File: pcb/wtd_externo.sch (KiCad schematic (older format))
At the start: 2 parts, among them U4 STWD100

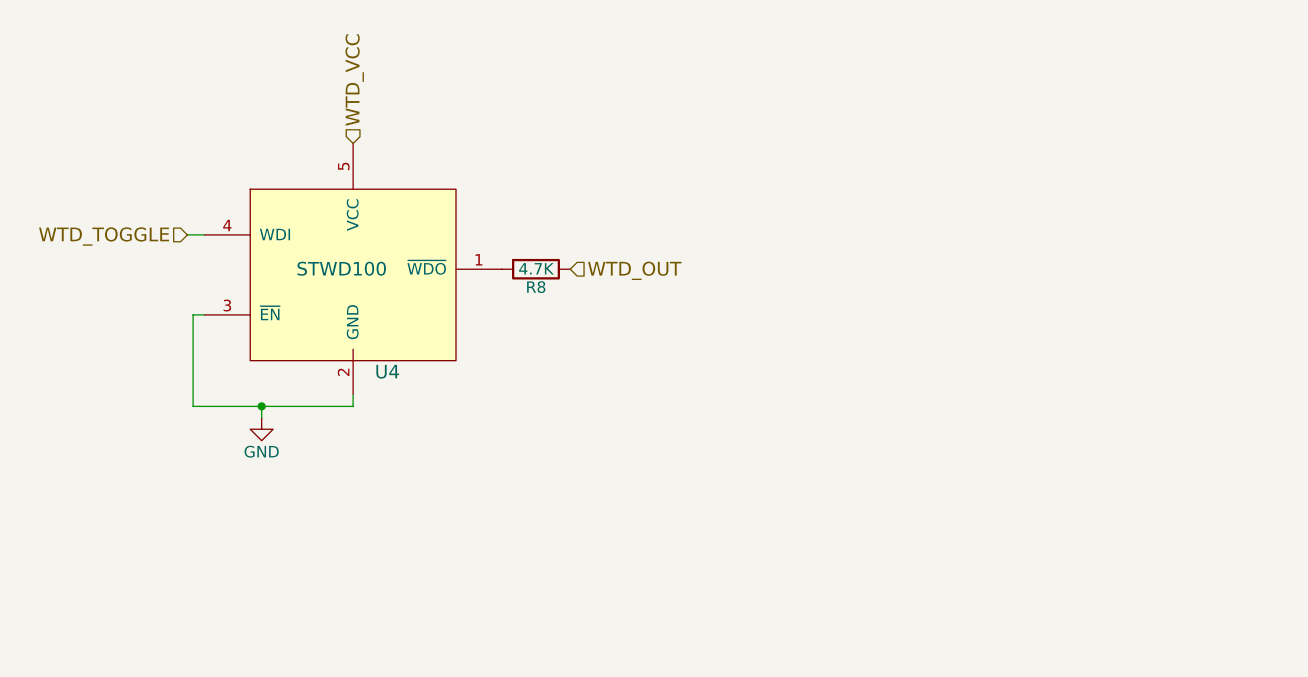
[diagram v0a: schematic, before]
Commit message: Clean up Kicad and TCC
Some changes in the
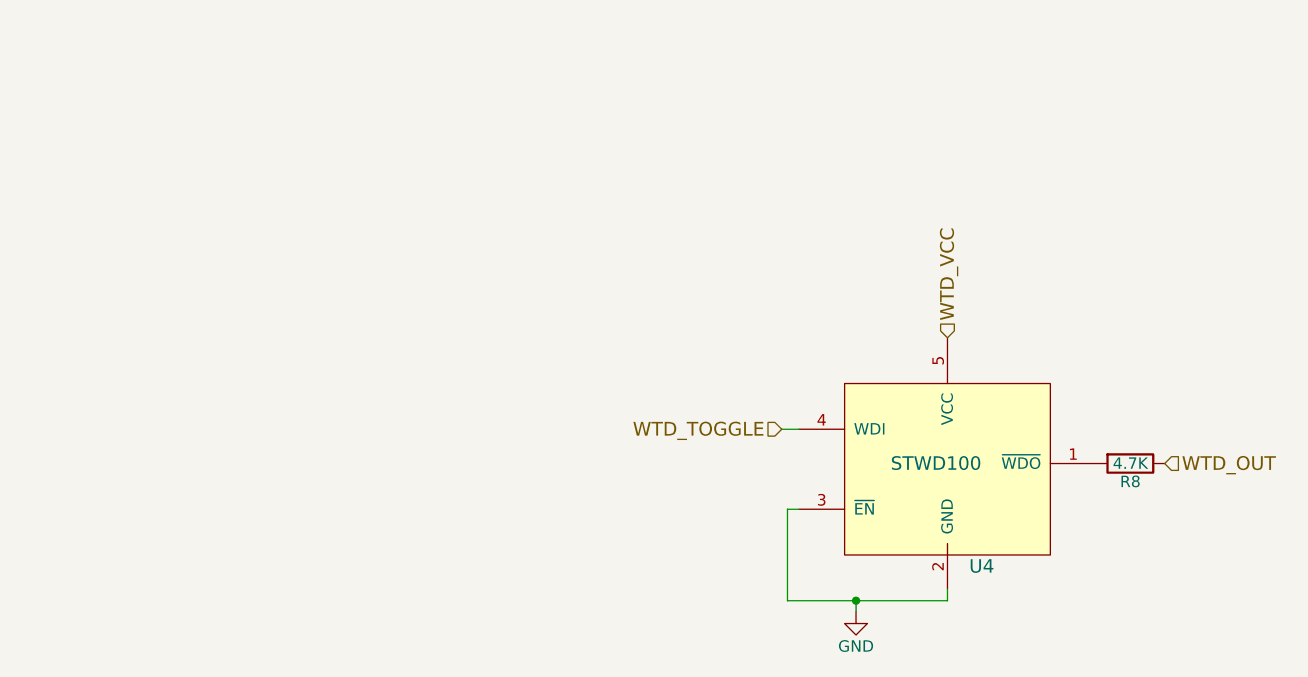
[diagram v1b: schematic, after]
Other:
- moved on the sheet: R8, U4
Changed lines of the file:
@@
 encoding utf-8
 Sheet 4 10
-Title ""
+Title "Watchdog Schematic"
 Date ""
-Rev ""
-Comp ""
+Rev "1"
+Comp "Universidade de Brasília - Campus Gama"
 Comment1 ""
 Comment2 ""
@@
 L stwd100:STWD100 U4
 U 1 1 5B1D7F0F
-P 3550 3450
-F 0 "U4" H 4050 3400 59  0000 C CNN
-F 1 "STWD100" H 3850 3850 59  0000 C CNN
-F 2 "TO_SOT_Packages_SMD:SOT-23-5" H 3550 3450 59  0001 C CNN
-F 3 "https://www.digikey.com/product-detail/en/stmicroelectronics/STWD100NYWY3F/497-10058-1-ND/2175107" H 3550 3450 59  0001 C CNN
-	1    3550 3450
+P 6150 4300
+F 0 "U4" H 6650 4250 59  0000 C CNN
+F 1 "STWD100" H 6450 4700 59  0000 C CNN
+F 2 "TO_SOT_Packages_SMD:SOT-23-5" H 6150 4300 59  0001 C CNN
+F 3 "https://www.digikey.com/product-detail/en/stmicroelectronics/STWD100NYWY3F/497-10058-1-ND/2175107" H 6150 4300 59  0001 C CNN
+	1    6150 4300
 	1    0    0    -1
 $EndComp
-Text HLabel 4850 3050 2    60   Input ~ 0
+Text HLabel 7450 3900 2    60   Input ~ 0
 WTD_OUT
-Text HLabel 3900 2500 1    60   Input ~ 0
+Text HLabel 6500 3350 1    60   Input ~ 0
 WTD_VCC
 $Comp
 L Device:R R8
 U 1 1 5B1D8509
-P 4700 3050
-F 0 "R8" V 4780 3050 50  0000 C CNN
-F 1 "4.7K" V 4700 3050 50  0000 C CNN
-F 2 "Resistors_SMD:R_1206" V 4630 3050 50  0001 C CNN
-F 3 "https://www.digikey.com/product-detail/en/te-connectivity-passive-product/CRGCQ1206J4K7/A130181CT-ND/8578013" H 4700 3050 50  0001 C CNN
-	1    4700 3050
+P 7300 3900
+F 0 "R8" V 7380 3900 50  0000 C CNN
+F 1 "4.7K" V 7300 3900 50  0000 C CNN
+F 2 "Resistors_SMD:R_1206" V 7230 3900 50  0001 C CNN
+F 3 "https://www.digikey.com/product-detail/en/te-connectivity-passive-product/CRGCQ1206J4K7/A130181CT-ND/8578013" H 7300 3900 50  0001 C CNN
+	1    7300 3900
 	0    1    1    0
 $EndComp
 Wire Wire Line
-	3900 3650 3900 3600
+	6500 4500 6500 4450
 Wire Wire Line
-	3200 3650 3500 3650
+	5800 4500 6100 4500
 Wire Wire Line
-	3250 3250 3200 3250
+	5850 4100 5800 4100
 Wire Wire Line
-	3200 3250 3200 3650
+	5800 4100 5800 4500
 $Comp
 L power:GND #PWR07
 U 1 1 5B1D859F
-P 3500 3700
-F 0 "#PWR07" H 3500 3450 50  0001 C CNN
-F 1 "GND" H 3500 3550 50  0000 C CNN
-F 2 "" H 3500 3700 50  0001 C CNN
-F 3 "" H 3500 3700 50  0001 C CNN
-	1    3500 3700
+P 6100 4550
+F 0 "#PWR07" H 6100 4300 50  0001 C CNN
+F 1 "GND" H 6100 4400 50  0000 C CNN
+F 2 "" H 6100 4550 50  0001 C CNN
+F 3 "" H 6100 4550 50  0001 C CNN
+	1    6100 4550
 	1    0    0    -1
 $EndComp
 Wire Wire Line
-	3500 3700 3500 3650
-Connection ~ 3500 3650
-Text HLabel 3175 2900 0    60   Input ~ 0
+	6100 4550 6100 4500
+Connection ~ 6100 4500
+Text HLabel 5775 3750 0    60   Input ~ 0
 WTD_TOGGLE
 Wire Wire Line
-	3175 2900 3250 2900
+	5775 3750 5850 3750
 Wire Wire Line
-	3500 3650 3900 3650
+	6100 4500 6500 4500
 $EndSCHEMATC
